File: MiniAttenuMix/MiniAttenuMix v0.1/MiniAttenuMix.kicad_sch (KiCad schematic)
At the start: 37 parts, among them U1 TL072, U2 TL072, U3 TL074

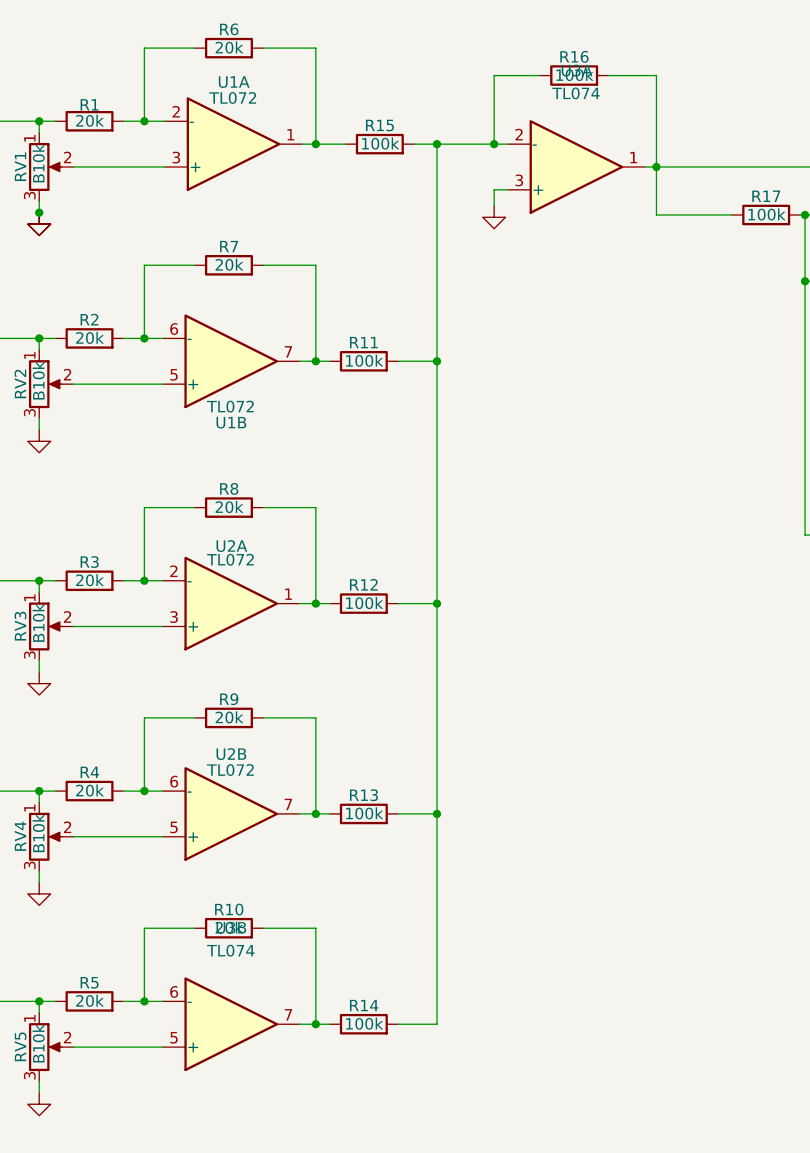
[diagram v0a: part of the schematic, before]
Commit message: Added v0.2 gerbers
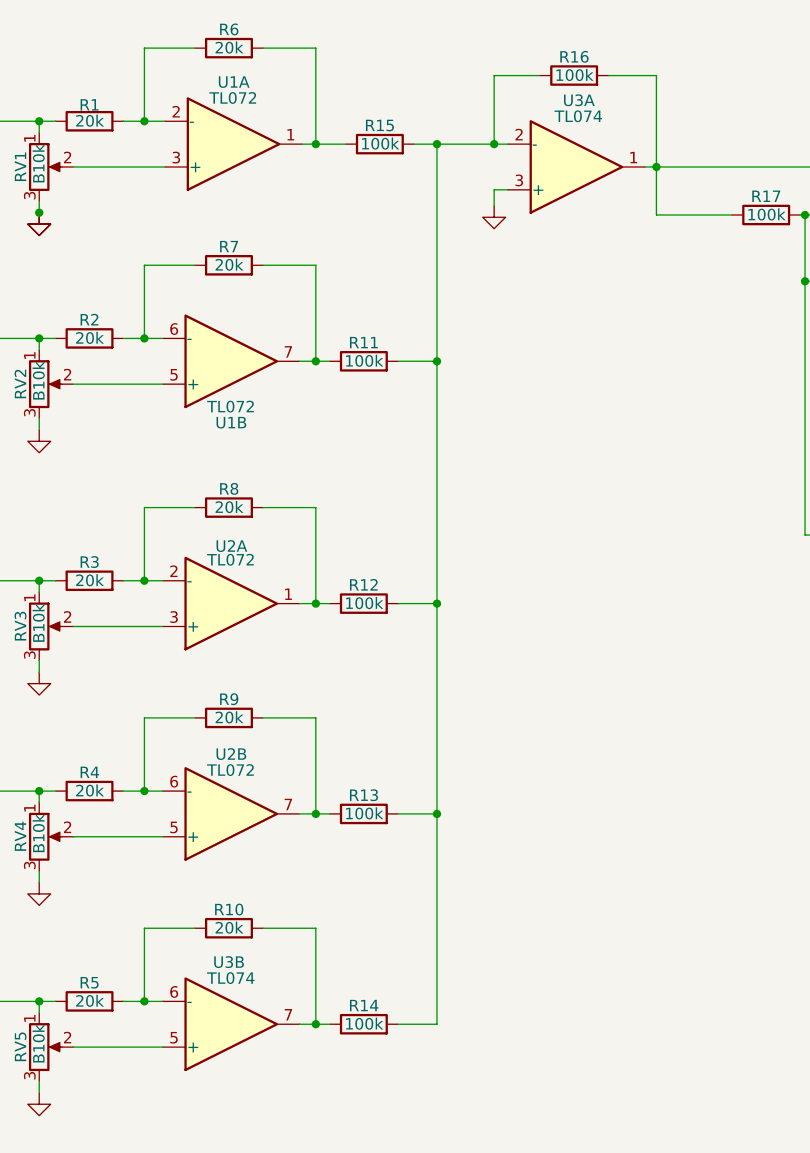
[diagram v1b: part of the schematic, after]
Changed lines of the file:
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@@
   )
   (symbol (lib_id "Amplifier_Operational:TL074") (at 123.698 39.878 0) (mirror x) (unit 1)
-    (in_bom yes) (on_board yes) (fields_autoplaced)
-    (property "Reference" "U3" (id 0) (at 123.698 29.21 0))
-    (property "Value" "TL074" (id 1) (at 123.698 31.75 0))
+    (in_bom yes) (on_board yes)
+    (property "Reference" "U3" (id 0) (at 123.952 32.512 0))
+    (property "Value" "TL074" (id 1) (at 123.952 34.29 0))
     (property "Footprint" "Package_SO:SOIC-14_3.9x8.7mm_P1.27mm" (id 2) (at 122.428 42.418 0)
       (effects (font (size 1.27 1.27)) hide)
@@
   )
   (symbol (lib_id "Amplifier_Operational:TL074") (at 85.344 135.128 0) (mirror x) (unit 2)
-    (in_bom yes) (on_board yes) (fields_autoplaced)
-    (property "Reference" "U3" (id 0) (at 85.344 124.46 0))
-    (property "Value" "TL074" (id 1) (at 85.344 127 0))
+    (in_bom yes) (on_board yes)
+    (property "Reference" "U3" (id 0) (at 85.09 128.27 0))
+    (property "Value" "TL074" (id 1) (at 85.344 130.048 0))
     (property "Footprint" "Package_SO:SOIC-14_3.9x8.7mm_P1.27mm" (id 2) (at 84.074 137.668 0)
       (effects (font (size 1.27 1.27)) hide)
